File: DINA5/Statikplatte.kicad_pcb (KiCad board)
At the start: 2 copper layers, 100 x 100 mm, 32 parts, among them J1 VIN, J10 HV, J2 GND, J3 GND, J4 GND, J5 GND, J6 GND, J7 HV, J8 HV, J9 HV

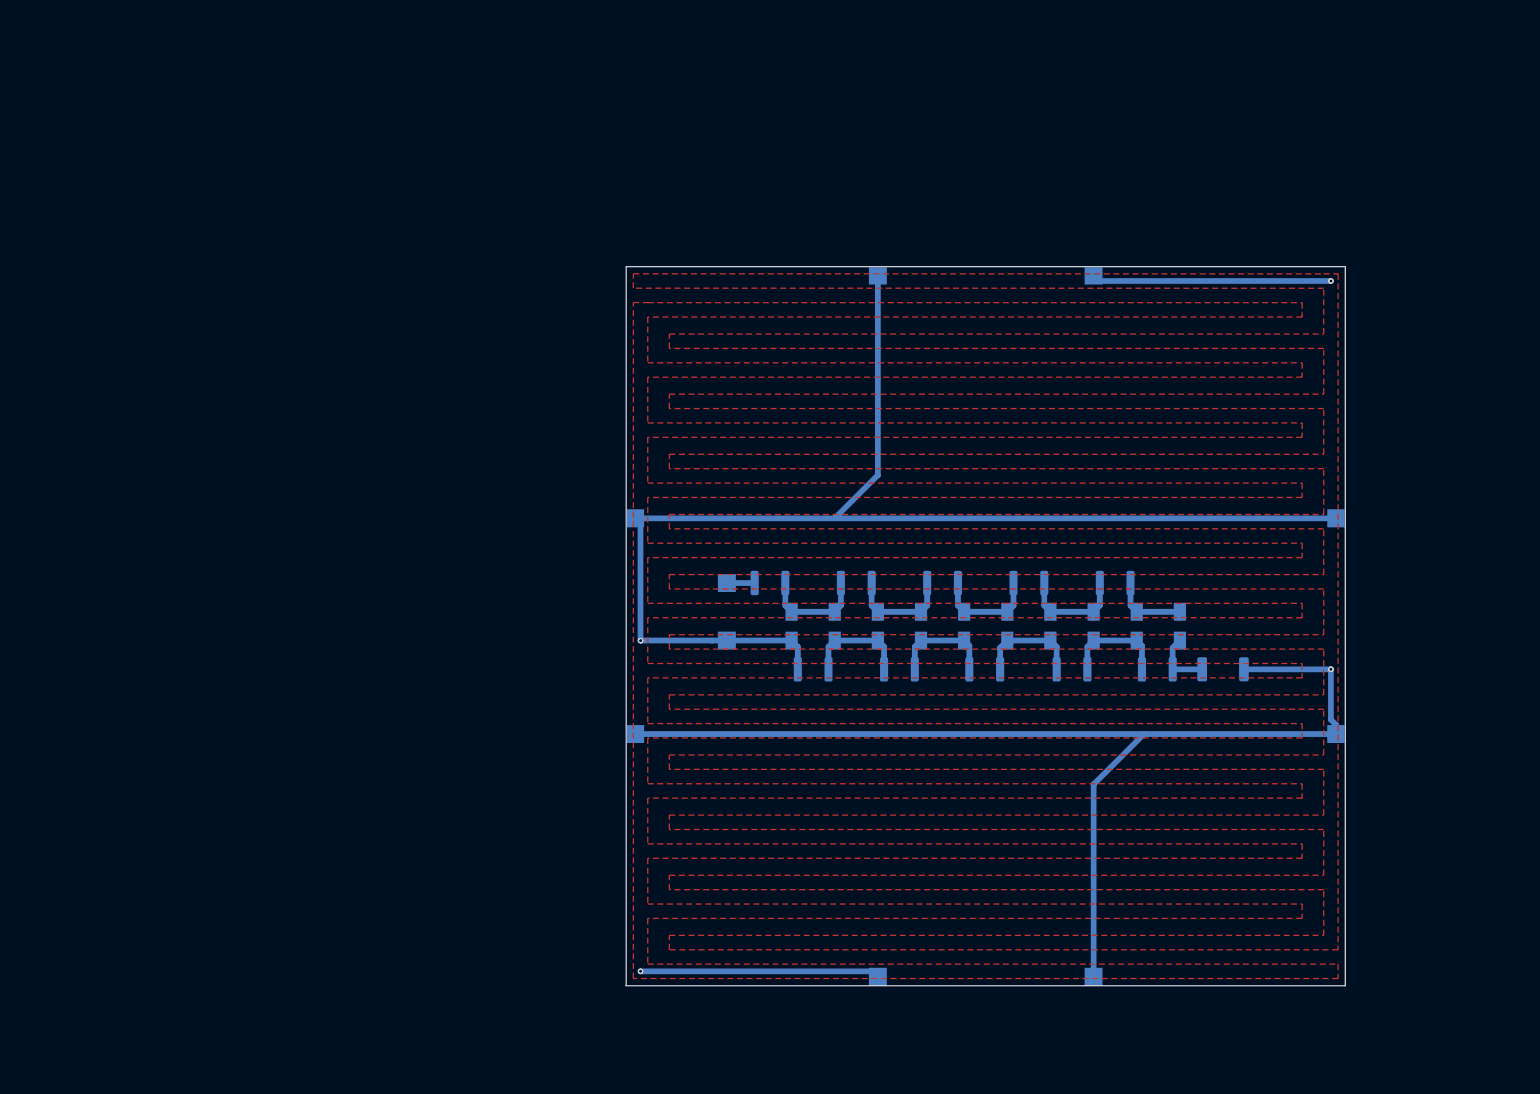
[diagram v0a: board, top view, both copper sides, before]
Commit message: added DINA5 files
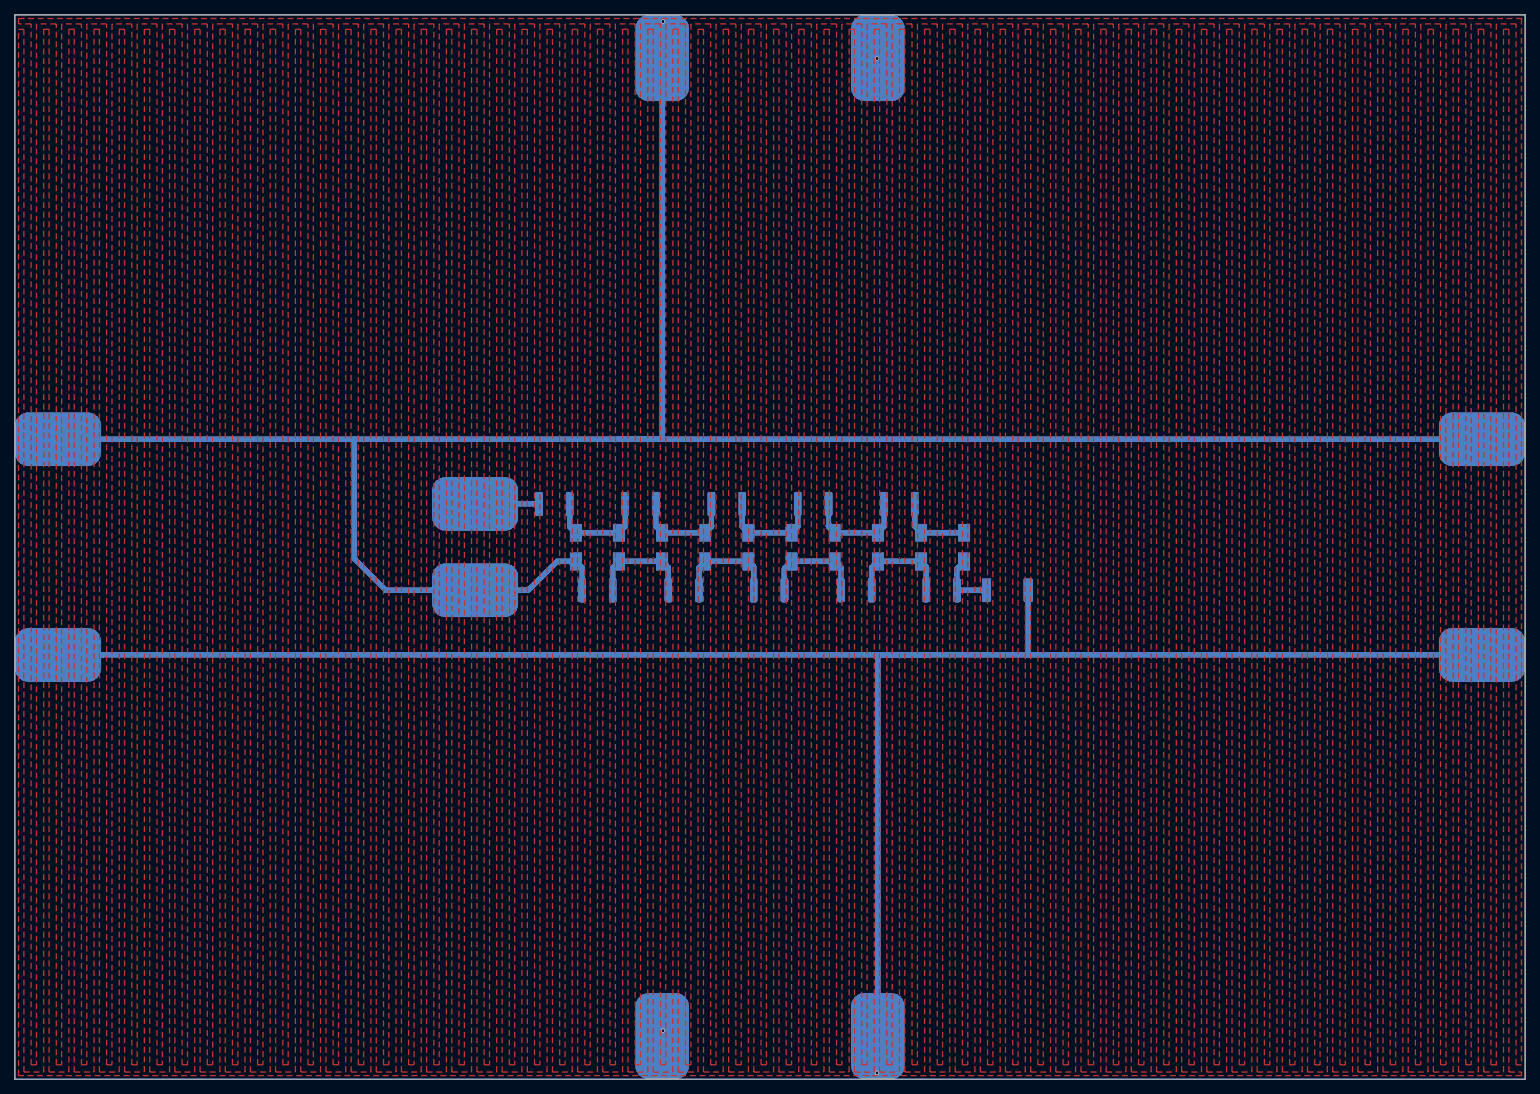
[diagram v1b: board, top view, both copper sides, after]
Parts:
- removed G***: LOGO, otter:otter_small1
- J1, J10, J2, J3, J4, J5, J6, J7, J8, J9: footprint TestPoint:TestPoint_Pad_2.5x2.5mm -> otter:Pads7.5x12
- moved J10 81.0 mm to (21.0, 104.0)
- moved J6 81.0 mm to (21.0, 74.0)
- moved J5 42.6 mm to (105.0, 21.0), turned to 270 degrees
- moved J8 42.6 mm to (135.0, 21.0), turned to 90 degrees
- moved J1 36.7 mm to (79.0, 83.0)
- moved J3 35.7 mm to (79.0, 95.0)
- moved C6 32.0 mm to (119.9, 95.0)
- moved C1 32.0 mm to (90.0, 83.0)
- moved C10 32.0 mm to (143.9, 95.0)
- moved C2 32.0 mm to (96.0, 95.0)
- moved C3 32.0 mm to (102.0, 83.0)
- moved C4 32.0 mm to (108.0, 95.0)
- moved C5 32.0 mm to (114.0, 83.0)
- moved C7 32.0 mm to (126.0, 83.0)
- moved C8 32.0 mm to (132.0, 95.0)
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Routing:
- net /GND: track 209.7 -> 312.2 mm
- net /HV: track 188.9 -> 267.2 mm
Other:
- board size 100 x 100 mm -> 210 x 148 mm
